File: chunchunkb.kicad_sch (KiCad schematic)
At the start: 124 parts, among them J1 BATT, J2 OLED, SW1 SW_Push, SW10 SW_Push, SW11 SW_Push, SW12 SW_Push, SW13 SW_Push, SW14 SW_Push, SW15 SW_Push, SW16 SW_Push, SW17 SW_Push, SW18 SW_Push, SW19 SW_Push, SW2 SW_Push, SW20 SW_Push, SW21 SW_Push, SW22 SW_Push, SW23 SW_Push, SW24 SW_Push, SW25 SW_Push, SW26 SW_Push, SW27 SW_Push, SW28 SW_Push, SW29 SW_Push, SW3 SW_Push, SW30 SW_Push, SW31 EC11, SW32 SW_Push, SW33 SW_Push, SW34 SW_Push, SW35 SW_Push, SW36 SW_Push, SW4 SW_Push, SW5 SW_Push, SW6 SW_Push, SW7 SW_Push, SW8 SW_Push, SW9 SW_Push

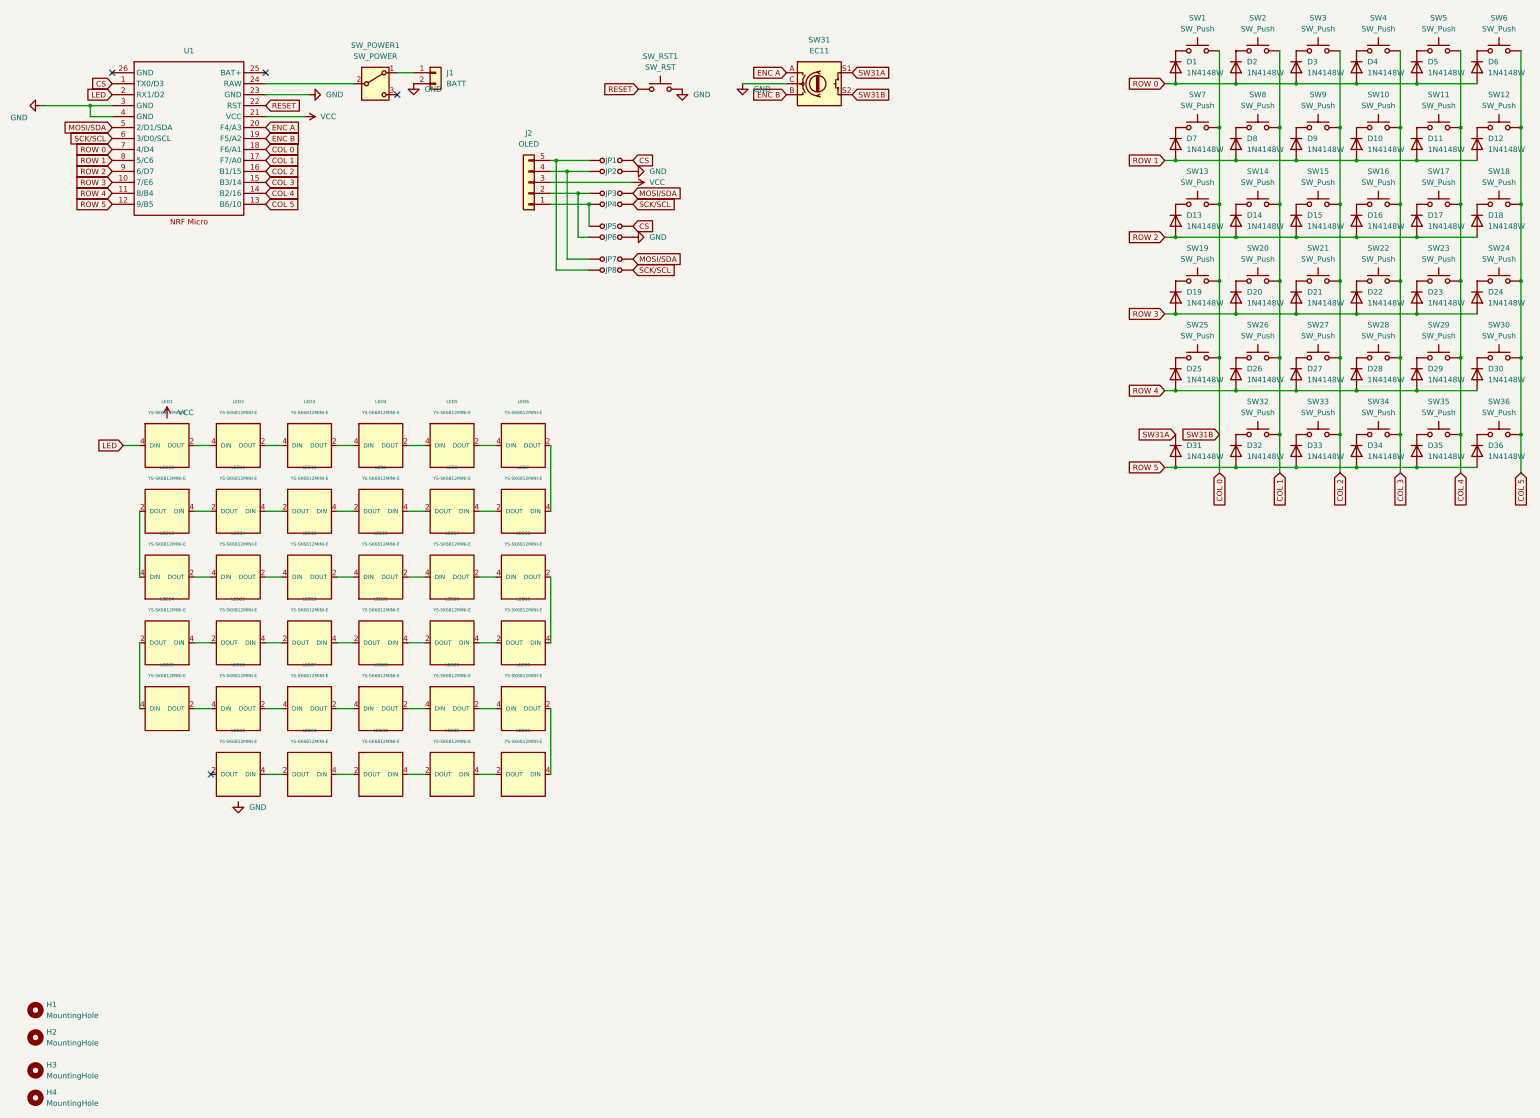
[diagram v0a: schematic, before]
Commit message: wip
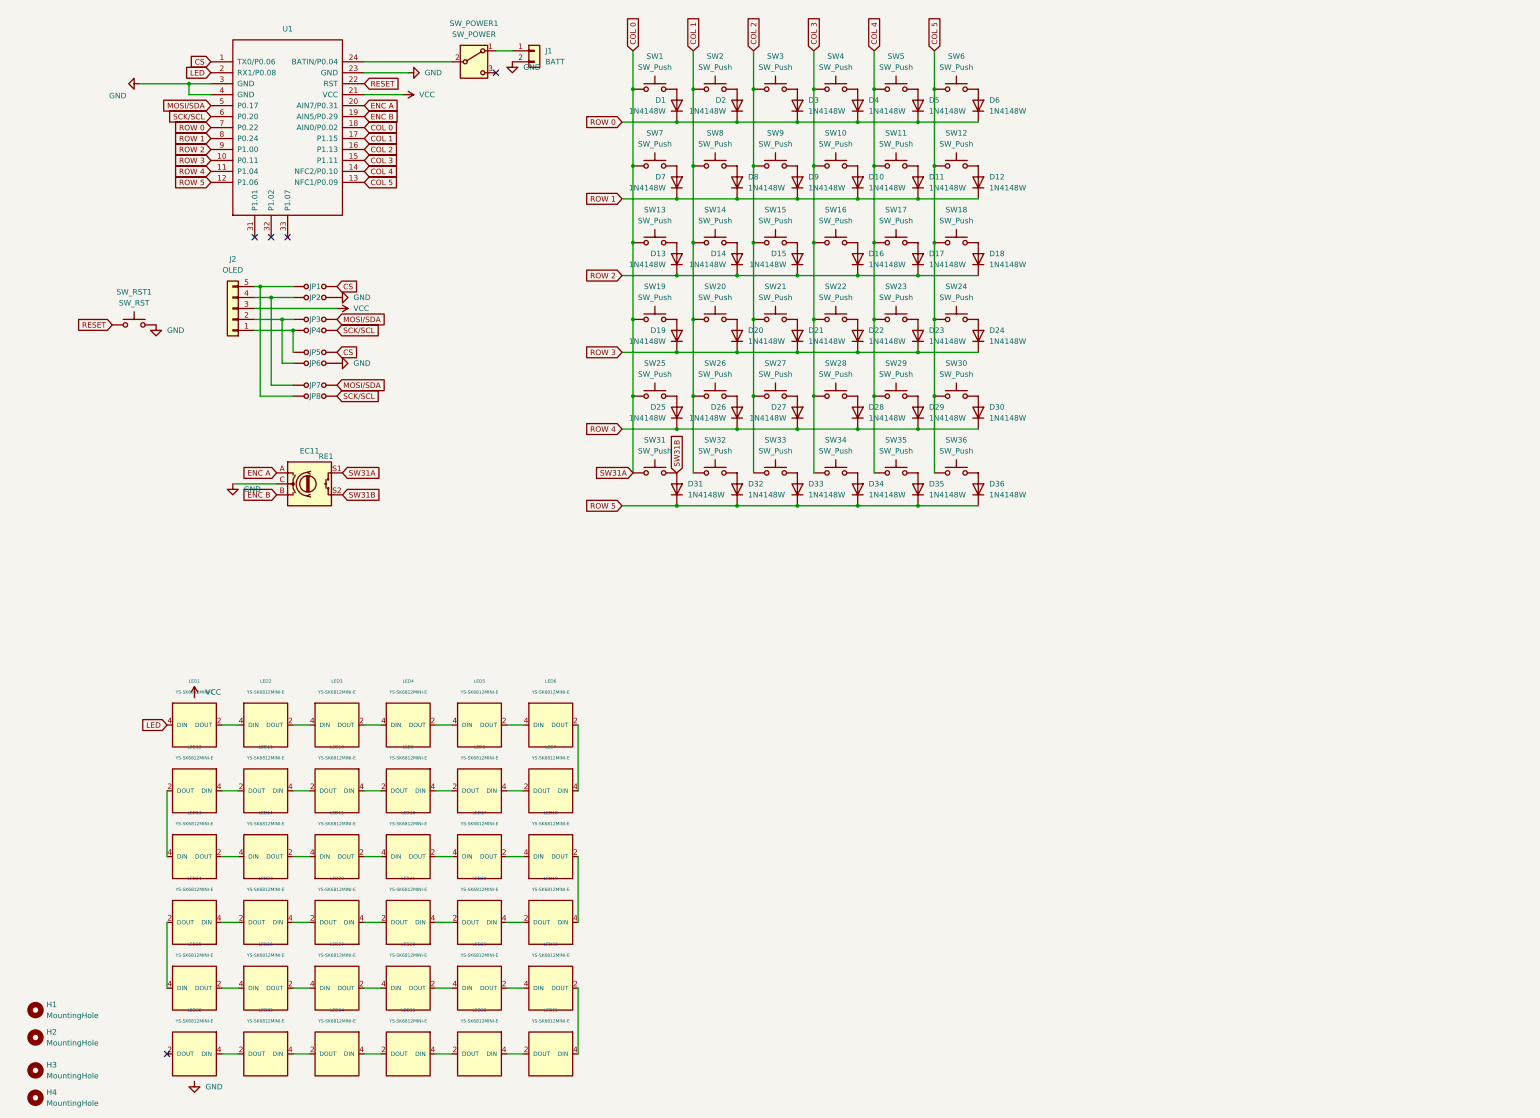
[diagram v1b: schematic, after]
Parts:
- added LED36: YS-SK6812MINI-E, chunchunkb:YS-SK6812MINI-E, symbol kbd:YS-SK6812MINI-E
- added SW31: SW_Push, chunchunkb:MX-1U-Hotswap, symbol Switch:SW_Push
- U1: footprint chunchunkb:ProMicro_DUAL -> chunchunkb:ProMicro_R; symbol Keyboard_CS:NRF_micro_jumper -> chunchunkb:nice_nano
- renumbered SW31 to RE1
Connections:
- net COL 0: now also RE1.S1, SW1.1, SW13.1, SW19.1, SW25.1, SW7.1, SW31.1; no longer RE1.S2, SW1.2, SW13.2, SW19.2, SW25.2, SW7.2
- net COL 1: now also SW14.1, SW2.1, SW20.1, SW26.1, SW32.1, SW8.1; no longer SW14.2, SW2.2, SW20.2, SW26.2, SW32.2, SW8.2
- net COL 2: now also SW15.1, SW21.1, SW27.1, SW3.1, SW33.1, SW9.1; no longer SW15.2, SW21.2, SW27.2, SW3.2, SW33.2, SW9.2
- net COL 3: now also SW10.1, SW16.1, SW22.1, SW28.1, SW34.1, SW4.1; no longer SW10.2, SW16.2, SW22.2, SW28.2, SW34.2, SW4.2
- net COL 4: now also SW11.1, SW17.1, SW23.1, SW29.1, SW35.1, SW5.1; no longer SW11.2, SW17.2, SW23.2, SW29.2, SW35.2, SW5.2
- net COL 5: now also SW12.1, SW18.1, SW24.1, SW30.1, SW36.1, SW6.1; no longer SW12.2, SW18.2, SW24.2, SW30.2, SW36.2, SW6.2
- net GND: now also LED36.3 (GND)
- net ROW 0: now also D1.1 (K), D2.1 (K), D3.1 (K), D4.1 (K), D5.1 (K), D6.1 (K); no longer D1.2 (A), D2.2 (A), D3.2 (A), D4.2 (A), D5.2 (A), D6.2 (A)
- net ROW 1: now also D10.1 (K), D11.1 (K), D12.1 (K), D7.1 (K), D8.1 (K), D9.1 (K); no longer D10.2 (A), D11.2 (A), D12.2 (A), D7.2 (A), D8.2 (A), D9.2 (A)
- net ROW 2: now also D13.1 (K), D14.1 (K), D15.1 (K), D16.1 (K), D17.1 (K), D18.1 (K); no longer D13.2 (A), D14.2 (A), D15.2 (A), D16.2 (A), D17.2 (A), D18.2 (A)
- net ROW 3: now also D19.1 (K), D20.1 (K), D21.1 (K), D22.1 (K), D23.1 (K), D24.1 (K); no longer D19.2 (A), D20.2 (A), D21.2 (A), D22.2 (A), D23.2 (A), D24.2 (A)
- net ROW 4: now also D25.1 (K), D26.1 (K), D27.1 (K), D28.1 (K), D29.1 (K), D30.1 (K); no longer D25.2 (A), D26.2 (A), D27.2 (A), D28.2 (A), D29.2 (A), D30.2 (A)
- net ROW 5: now also D31.1 (K), D32.1 (K), D33.1 (K), D34.1 (K), D35.1 (K), D36.1 (K); no longer D31.2 (A), D32.2 (A), D33.2 (A), D34.2 (A), D35.2 (A), D36.2 (A)
- net VCC: now also LED36.1 (VDD)
- net at LED35.2 (DOUT): now also LED36.4 (DIN)
- removed net SW31A: D31.1 (K), RE1.S1
- new net: D14.2 (A), SW14.2
- new net: D25.2 (A), SW25.2
- new net: D23.2 (A), SW23.2
- new net: D30.2 (A), SW30.2
- new net: D4.2 (A), SW4.2
- new net: D10.2 (A), SW10.2
- new net: D27.2 (A), SW27.2
- new net: D8.2 (A), SW8.2
- new net: D17.2 (A), SW17.2
- new net: D16.2 (A), SW16.2
- new net: D6.2 (A), SW6.2
- new net: D13.2 (A), SW13.2
- new net: D26.2 (A), SW26.2
- new net: D5.2 (A), SW5.2
- new net: D24.2 (A), SW24.2
- new net: D35.2 (A), SW35.2
- new net: D36.2 (A), SW36.2
- new net: D32.2 (A), SW32.2
- new net: D3.2 (A), SW3.2
- new net: D12.2 (A), SW12.2
- new net: D19.2 (A), SW19.2
- new net: D21.2 (A), SW21.2
- new net: D7.2 (A), SW7.2
- new net: D28.2 (A), SW28.2
- new net: D33.2 (A), SW33.2
- new net: D20.2 (A), SW20.2
- new net: D2.2 (A), SW2.2
- new net: D11.2 (A), SW11.2
- new net: D29.2 (A), SW29.2
- new net: D15.2 (A), SW15.2
- new net: D9.2 (A), SW9.2
- new net: D18.2 (A), SW18.2
- new net: D22.2 (A), SW22.2
- new net: D1.2 (A), SW1.2
- new net: D34.2 (A), SW34.2
- new net SW31B: D31.2 (A), RE1.S2, SW31.2
- no-connect marks 4 -> 5
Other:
- moved on the sheet: D1, D10, D11, D12, D13, D14, D15, D16, D17, D18, D19, D2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
